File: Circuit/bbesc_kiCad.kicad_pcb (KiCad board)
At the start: 2 copper layers, 90.8 x 78.7 mm, 70 parts, among them J1 CONN_01X02, Q1 Q_NMOS_GDS, Q2 Q_NMOS_GDS, Q3 Q_NMOS_GDS, Q4 Q_NMOS_GDS, Q5 Q_NMOS_GDS, Q6 Q_NMOS_GDS, U1 teensy_3-2, U2 IR2101, U3 IR2101, U4 IR2101, U5 INA21x, U6 LM7805, U7 INA21x, U8 TJA1051T-SN65HVD230D

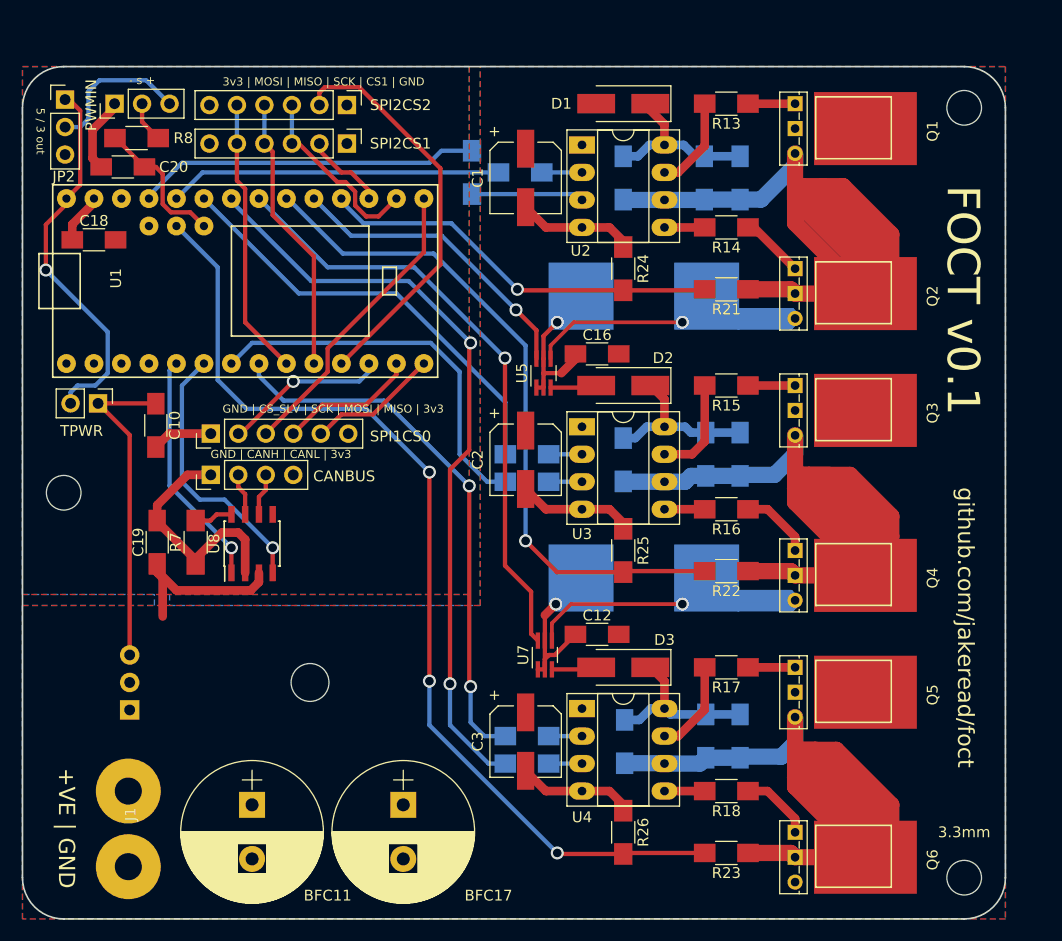
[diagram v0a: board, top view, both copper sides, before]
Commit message: board v0.2
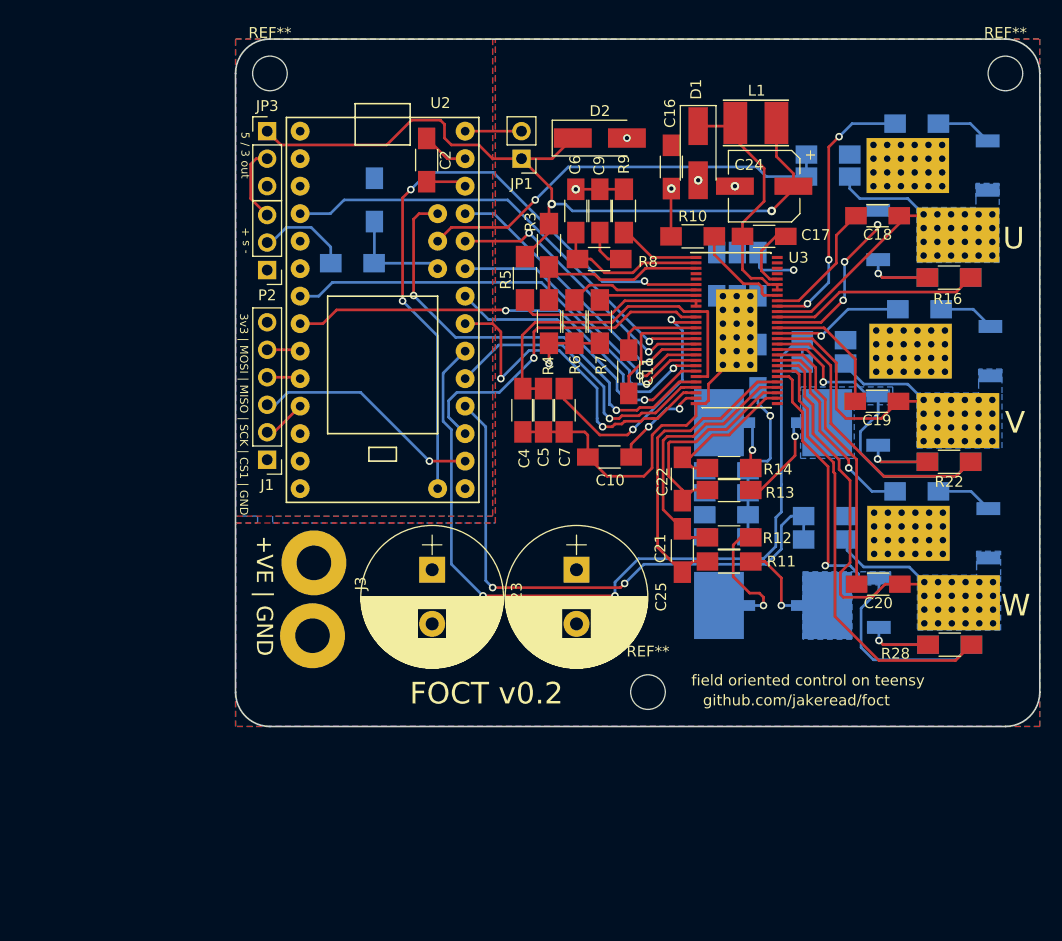
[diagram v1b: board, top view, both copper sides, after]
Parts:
- removed 3.3mm, ? (x2): MountingHole_3.2mm_M3, Mounting_Holes:MountingHole_3.2mm_M3
- removed BFC11, BFC17: 2000uF, Capacitors_ThroughHole:CP_Radial_D13.0mm_P5.00mm
- removed C1: 56uF, Capacitors_SMD:CP_Elec_6.3x7.7
- removed C8: 10uF, Capacitors_SMD:C_1206_HandSoldering
- removed CANBUS: CONN_01X04, Pin_Headers:Pin_Header_Straight_1x04_Pitch2.54mm
- removed D3: 1N4001, Diodes_SMD:D_SMA_Handsoldering
- removed JP2: JUMPER3, Pin_Headers:Pin_Header_Straight_1x03_Pitch2.54mm
- removed PWMIN: CONN_01X03, Pin_Headers:Pin_Header_Straight_1x03_Pitch2.54mm
- removed R1: 220R, Resistors_SMD:R_1206_HandSoldering
- removed SPI1CS0, SPI2CS1, SPI2CS2: CONN_01X06, Pin_Headers:Pin_Header_Straight_1x06_Pitch2.54mm
- removed TPWR: JUMPER, Pin_Headers:Pin_Header_Straight_1x02_Pitch2.54mm
- removed U1: teensy_3-2, teensy_3-2_bottomLess:Teensy3.2-bottomLess
- removed U4: IR2101, Housings_DIP:DIP-8_W7.62mm_Socket_LongPads
- removed U5, U7: INA21x, TO_SOT_Packages_SMD:SOT-363_SC-70-6_Handsoldering
- removed U6: LM7805, TO_SOT_Packages_THT:TO-220_Horizontal
- removed U8: TJA1051T-SN65HVD230D, Housings_SOIC:SOIC-8_3.9x4.9mm_Pitch1.27mm
- added C11: 22nF, Capacitors_SMD:C_1206_HandSoldering, F.Cu at (133.2, 97.8)
- added C17: 100nF, Capacitors_SMD:C_1206_HandSoldering, F.Cu at (145.7, 85.3)
- added C21: 2.2nF, Capacitors_SMD:C_1206_HandSoldering, F.Cu at (138.2, 114.3)
- added C22: 2.2nF, Capacitors_SMD:C_1206_HandSoldering, F.Cu at (138.2, 107.7)
- added C23: 2000uF, Capacitors_ThroughHole:CP_Radial_D13.0mm_P5.00mm, F.Cu at (115.1, 116.1)
- added C24: 100uF, Capacitors_SMD:CP_Elec_6.3x7.7, F.Cu at (145.7, 80.6)
- added C25: 2000uF, Capacitors_ThroughHole:CP_Radial_D13.0mm_P5.00mm, F.Cu at (128.4, 116.1)
- added C26: 10uF, Capacitors_SMD:C_1206_HandSoldering, B.Cu at (145.2, 97.3)
- added C29: 10uF, Capacitors_SMD:C_1206_HandSoldering, B.Cu at (145.2, 88.8)
- added C30: 10uF, Capacitors_SMD:C_1206_HandSoldering, B.Cu at (143.3, 88.8)
- added C31: 10uF, Capacitors_SMD:C_1206_HandSoldering, B.Cu at (141.4, 88.8)
- added J3: CONN_01X02, Wire_Connections_Bridges:WireConnection_2.50mmDrill_LargePad, F.Cu at (104.1, 125.6)
- added JP1: JUMPER, Pin_Headers:Pin_Header_Straight_1x02_Pitch2.54mm, F.Cu at (123.3, 78.1)
- added JP3: JUMPER3, Pin_Headers:Pin_Header_Straight_1x03_Pitch2.54mm, F.Cu at (99.8, 75.6)
- added L1: 22uH, Inductors:Inductor_Taiyo-Yuden_NR-40xx_HandSoldering, F.Cu at (145.0, 74.8)
- added P2: CONN_01X03, Pin_Headers:Pin_Header_Straight_1x03_Pitch2.54mm, F.Cu at (99.8, 88.4)
- added R10: 1M, Resistors_SMD:R_1206_HandSoldering, F.Cu at (139.1, 85.3)
- added R11: 100R, Resistors_SMD:R_1206_HandSoldering, F.Cu at (142.5, 115.3)
- added R12: 100R, Resistors_SMD:R_1206_HandSoldering, F.Cu at (142.5, 113.1)
- added R19: 39K, Resistors_SMD:R_1206_HandSoldering, B.Cu at (151.6, 79.8)
- added R20: 5K6, Resistors_SMD:R_1206_HandSoldering, B.Cu at (151.6, 77.7)
- added R27: 4R7, Resistors_SMD:R_1206_HandSoldering, B.Cu at (159.8, 108.8)
- added R29: 39k, Resistors_SMD:R_1206_HandSoldering, B.Cu at (162.9, 123.0)
- added R30: 39K, Resistors_SMD:R_1206_HandSoldering, B.Cu at (151.4, 113.3)
- added R31: 5K6, Resistors_SMD:R_1206_HandSoldering, B.Cu at (151.4, 111.1)
- added REF**: MountingHole_3.2mm_M3_ISO14580, Mounting_Holes:MountingHole_3.2mm_M3_ISO14580, F.Cu at (168.0, 70.2)
- added REF**: MountingHole_3.2mm_M3_ISO14580, Mounting_Holes:MountingHole_3.2mm_M3_ISO14580, F.Cu at (100.1, 70.2)
- added REF**: MountingHole_3.2mm_M3_ISO14580, Mounting_Holes:MountingHole_3.2mm_M3_ISO14580, F.Cu at (135.0, 127.4)
- C10: value 10uF -> 2.2uF
- C12: value 0.1uF -> 10uF; moved to B.Cu
- C16: value 0.1uF -> 10uF
- C18, C19, C20: value 10uF -> 220nF
- C2: value 56uF -> 10uF; footprint Capacitors_SMD:CP_Elec_6.3x7.7 -> Capacitors_SMD:C_1206_HandSoldering
- C3: value 56uF -> 10uF; footprint Capacitors_SMD:CP_Elec_6.3x7.7 -> Capacitors_SMD:C_1206_HandSoldering; moved to B.Cu
- C4: value 10uF -> 2.2uF; moved to F.Cu
- C5, C7: value 0.1uF -> 2.2uF; moved to F.Cu
- C6: value 10uF -> 120pF; moved to F.Cu
- C9: value 0.1uF -> 6.8nF; moved to F.Cu
- D1: value 1N4001 -> DIODESCH
- D2: value 1N4001 -> TVS 5v
- J1: value CONN_01X02 -> CONN_01X06; footprint Wire_Connections_Bridges:WireConnection_2.50mmDrill_LargePad -> Pin_Headers:Pin_Header_Straight_1x06_Pitch2.54mm
- Q1, Q2, Q3, Q4, Q5, Q6: footprint TO-251_IPAK_Slammed:TO-251_IPAK_Vertical -> HTO-252:TO-252-2; moved to B.Cu
- R13, R14: value 4R7 -> 100R
- R15, R26: moved to B.Cu
- R17: value 4R7 -> 39k; moved to B.Cu
- R18: value 4R7 -> SHNT; footprint Resistors_SMD:R_1206_HandSoldering -> R_SHUNT_3920:R_SHUNT_3920; moved to B.Cu
- R2: value 220R -> 47R
- R21: value 39K -> 4R7; moved to B.Cu
- R22: value 39K -> 4R7
- R23: value 39K -> 39k; moved to B.Cu
- R24: value 5K6 -> SHNT; footprint Resistors_SMD:R_1206_HandSoldering -> R_SHUNT_3920:R_SHUNT_3920; moved to B.Cu
- R25: value 5K6 -> 39K; moved to B.Cu
- R28: value .001 -> 4R7; footprint R_SHUNT_3920:R_2816_HandSoldering -> Resistors_SMD:R_1206_HandSoldering; moved to F.Cu
- R3: value 220R -> 18k; moved to F.Cu
- R4, R6: value 220R -> 3k3; moved to F.Cu
- R5: value 220R -> 10k; moved to F.Cu
- R7: value 10K -> 3k3
- R8: value 47R -> 15k
- R9: value .001 -> 220k; footprint R_SHUNT_3920:R_2816_HandSoldering -> Resistors_SMD:R_1206_HandSoldering; moved to F.Cu
- U2: value IR2101 -> teensy_3-2; footprint Housings_DIP:DIP-8_W7.62mm_Socket_LongPads -> teensy_3-2_bottomLess:Teensy3.2-bottomLess
- U3: value IR2101 -> DRV_8302; footprint Housings_DIP:DIP-8_W7.62mm_Socket_LongPads -> HTSSOP-56:TSSOP-56_6.1x14mm_Pitch0.5mm
- moved C20 79.7 mm to (156.3, 117.4), turned to 180 degrees
- moved C18 72.4 mm to (156.2, 83.4), turned to 180 degrees
- moved C19 67.7 mm to (156.1, 100.5), turned to 180 degrees
- moved C3 52.0 mm to (109.7, 81.9)
- moved C9 49.5 mm to (130.6, 82.9)
- moved R26 49.1 mm to (151.3, 94.9), turned to 0 degrees
- moved R8 44.2 mm to (130.5, 87.4)
- moved R7 42.5 mm to (130.6, 93.2)
- moved R5 42.3 mm to (123.6, 89.2), turned to 90 degrees
- moved C10 42.0 mm to (131.4, 105.7), turned to 180 degrees
- moved R23 41.6 mm to (162.8, 106.1)
- moved R17 41.5 mm to (162.8, 89.1)
- moved R6 41.1 mm to (128.2, 93.2), turned to 90 degrees
- moved J1 39.7 mm to (99.8, 105.9), turned to 180 degrees
- moved R13 35.7 mm to (142.5, 108.7)
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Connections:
- C12 pad 1: GND -> VCC
- C12 pad 2: VCC -> GND
- C13 pad 1: PHASE_U -> VCC
- C13 pad 2: Net-(C13-Pad2) -> GND
- C14 pad 1: PHASE_V -> VCC
- C14 pad 2: Net-(C14-Pad2) -> GND
- C15 pad 1: PHASE_W -> VCC
- C15 pad 2: Net-(C15-Pad2) -> GND
- C18 pad 1: GND -> PHASE_U
- C18 pad 2: 3v3 -> Net-(C18-Pad2)
- C19 pad 1: VCC -> PHASE_V
- C19 pad 2: GND -> Net-(C19-Pad2)
- C2 pad 1: VCC -> GND
- C2 pad 2: GND -> 3v3
- C20 pad 1: GND -> PHASE_W
- C3 pad 1: VCC -> GND
- C3 pad 2: GND -> SIMPLE_INPUT
- C4 pad 1: PHASE_U -> Net-(C4-Pad1)
- C4 pad 2: Net-(C13-Pad2) -> GND
- C5 pad 1: PHASE_U -> Net-(C4-Pad1)
- C5 pad 2: Net-(C13-Pad2) -> GND
- C6 pad 1: PHASE_V -> Net-(C6-Pad1)
- C6 pad 2: Net-(C14-Pad2) -> GND
- C7 pad 1: PHASE_V -> Net-(C7-Pad1)
- C7 pad 2: Net-(C14-Pad2) -> GND
- C9 pad 1: PHASE_W -> Net-(C9-Pad1)
- C9 pad 2: Net-(C15-Pad2) -> GND
- D1 pad 1: Net-(C13-Pad2) -> Net-(C17-Pad1)
- D1 pad 2: VCC -> GND
- D2 pad 1: Net-(C14-Pad2) -> 5v
- D2 pad 2: VCC -> GND
- J1 pad 2: VCC -> CS2
- Q2 pad 3: Net-(Q2-Pad3) -> GND
- Q4 pad 3: Net-(Q4-Pad3) -> /H_V_LO
- Q6 pad 3: GND -> /H_W_LO
- R13 pad 1: Net-(Q1-Pad1) -> /SHNT_V_HI
- R13 pad 2: Net-(R13-Pad2) -> Net-(C22-Pad2)
- R14 pad 1: Net-(Q2-Pad1) -> /SHNT_V_LO
- R14 pad 2: Net-(R14-Pad2) -> Net-(C22-Pad1)
- R15 pad 1: Net-(Q3-Pad1) -> Net-(Q1-Pad1)
- R15 pad 2: Net-(R15-Pad2) -> DRV_HI_U
- R16 pad 1: Net-(Q4-Pad1) -> Net-(Q2-Pad1)
- R16 pad 2: Net-(R16-Pad2) -> DRV_LO_U
- R17 pad 1: Net-(Q5-Pad1) -> GND
- R17 pad 2: Net-(R17-Pad2) -> Net-(Q2-Pad1)
- R18 pad 1: Net-(Q6-Pad1) -> /H_V_LO
- R18 pad 2: Net-(R18-Pad2) -> GND
- R2 pad 1: Net-(R2-Pad1) -> SIMPLE_INPUT
- R2 pad 2: LO_U -> Net-(P2-Pad2)
- R21 pad 1: PHASE_U -> Net-(Q3-Pad1)
- R21 pad 2: V_SENS_U -> DRV_HI_V
- R22 pad 1: PHASE_V -> Net-(Q4-Pad1)
- R22 pad 2: V_SENS_V -> DRV_LO_V
- R23 pad 1: PHASE_W -> /H_V_LO
- R23 pad 2: V_SENS_W -> Net-(Q4-Pad1)
- R24 pad 1: GND -> /H_W_LO
- R24 pad 2: V_SENS_U -> GND
- R25 pad 1: GND -> PHASE_V
- R26 pad 1: GND -> V_SENS_V
- R26 pad 2: V_SENS_W -> GND
- R28 pad 1: Net-(Q4-Pad3) -> Net-(Q6-Pad1)
- R28 pad 2: GND -> DRV_LO_W
- R3 pad 2: HI_V -> 5v
- R4 pad 1: Net-(R4-Pad1) -> GND
- R4 pad 2: LO_V -> Net-(R3-Pad1)
- R5 pad 2: HI_W -> 5v
- R6 pad 1: Net-(R6-Pad1) -> GND
- R6 pad 2: LO_W -> Net-(R6-Pad2)
- R8 pad 1: Net-(C20-Pad2) -> Net-(C6-Pad1)
- R8 pad 2: Net-(P1-Pad2) -> Net-(C9-Pad1)
- R9 pad 1: Net-(Q2-Pad3) -> Net-(R9-Pad1)
- U2 pad 1: VCC -> Net-(U2-Pad1)
- U2 pad 2: Net-(R1-Pad1) -> EN_GATE
- U2 pad 3: Net-(R2-Pad1) -> CANTX
- U2 pad 4: GND -> CANRX
- U2 pad 5: Net-(R14-Pad2) -> MC_LO_V
- U2 pad 6: PHASE_U -> MC_HI_W
- U2 pad 7: Net-(R13-Pad2) -> MOSI2
- U2 pad 8: Net-(C13-Pad2) -> MISO2
- U3 pad 1: VCC -> Net-(R9-Pad1)
- U3 pad 2: Net-(R3-Pad1) -> Net-(C6-Pad1)
- U3 pad 3: Net-(R4-Pad1) -> Net-(R3-Pad1)
- U3 pad 4: GND -> Net-(U3-Pad4)
- U3 pad 5: Net-(R16-Pad2) -> Net-(U3-Pad5)
- U3 pad 6: PHASE_V -> DRV_FAULT
- U3 pad 7: Net-(R15-Pad2) -> Net-(R6-Pad2)
- U3 pad 8: Net-(C14-Pad2) -> Net-(R7-Pad2)
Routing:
- net PHASE_U: track 116.5 -> 27.4 mm
- net Net-(Q4-Pad3): track 84.0 -> 0.00 mm, vias 1 -> 0
- net Net-(Q2-Pad3): track 83.1 -> 0.00 mm, vias 1 -> 0
- net PHASE_V: track 99.6 -> 28.5 mm
- net LO_W: track 70.6 -> 0.00 mm, vias 2 -> 0
- net DRV_FAULT: track 0.00 -> 60.6 mm, vias 0 -> 3
- net PHASE_W: track 99.6 -> 43.4 mm
- net GND: track 102.1 -> 50.4 mm, vias 2 -> 6
- net HI_W: track 50.4 -> 0.00 mm, vias 2 -> 0
- net /H_W_LO: track 0.00 -> 44.7 mm, vias 0 -> 1
- net EN_GATE: track 0.00 -> 42.6 mm, vias 0 -> 1
- net MC_LO_V: track 0.00 -> 42.5 mm, vias 0 -> 1
- net MC_AREF: track 0.00 -> 42.2 mm, vias 0 -> 2
- net MC_HI_W: track 0.00 -> 41.7 mm, vias 0 -> 2
- net DRV_LO_W: track 0.00 -> 40.8 mm
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- added copper zone on B.Cu, net /H_V_LO
- added copper zone on B.Cu, net /H_W_LO
- added copper zone on B.Cu, net PHASE_U
- added copper zone on B.Cu, net PHASE_V
- added copper zone on B.Cu, net PHASE_W
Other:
- board size 90.8 x 78.7 mm -> 74.3 x 63.5 mm
- net class Default: clearance 0.15 -> 0.2; trace_width 0.4 -> 0.25; via_dia 1.2 -> 0.7; via_drill 0.8 -> 0.4
- net class Drive: trace_width 0.8 -> 0.25; via_dia 1.2 -> 0.7; via_drill 0.8 -> 0.4
- net class Phase: trace_width 1.5 -> 0.25; via_dia 1.2 -> 0.7; via_drill 0.8 -> 0.4
- net class Phase Measurement: trace_width 0.35 -> 0.4; via_dia 1.2 -> 0.7; via_drill 0.8 -> 0.4
- rule trace_clearance: 0.15 -> 0.2
- board text added: "FOCT v0.2"
- board text added: "U"
- board text added: "V"
- board text added: "W"
- board text added: "field oriented control on teensy"
- board text removed: "FOCT v0.1"
- board text removed: "GND | CANH | CANL | 3v3"
- board text removed: "GND | CS_SLV | SCK | MOSI | MISO | 3v3"
